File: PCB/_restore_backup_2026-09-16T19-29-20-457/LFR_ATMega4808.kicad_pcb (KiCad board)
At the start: 2 copper layers, 51.7 x 63.4 mm, 49 parts, among them J1 Conn_02x02_Odd_Even, J2 Conn_02x05_Odd_Even, J3 Conn_02x02_Counter_Clockwise, J4 Conn_02x02_Counter_Clockwise, J5 Conn_02x02_Counter_Clockwise, J6 Conn_02x03_Odd_Even, Q2 NMOS, Q3 NMOS, U1 ATmega4808-A, U5 MCP1700x-330xxTO

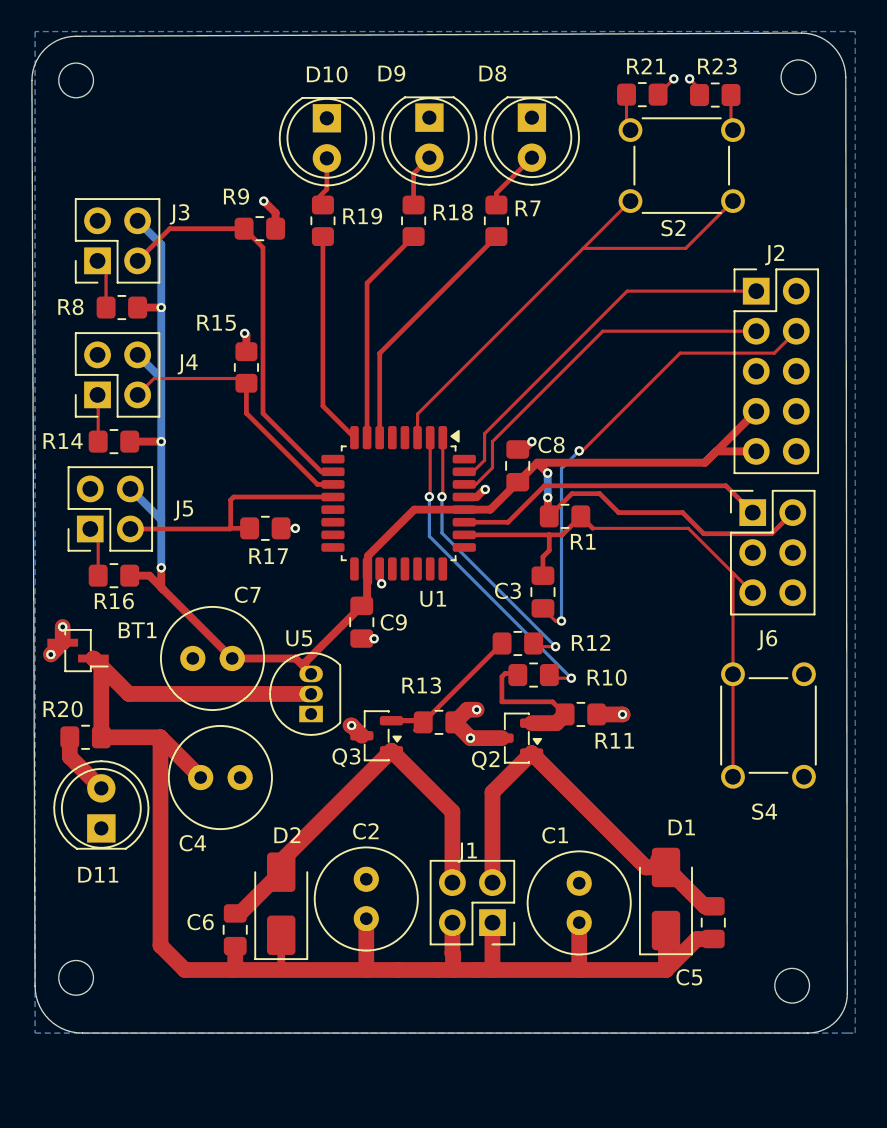
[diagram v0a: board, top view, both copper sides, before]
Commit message: Final touches, v1 is ready
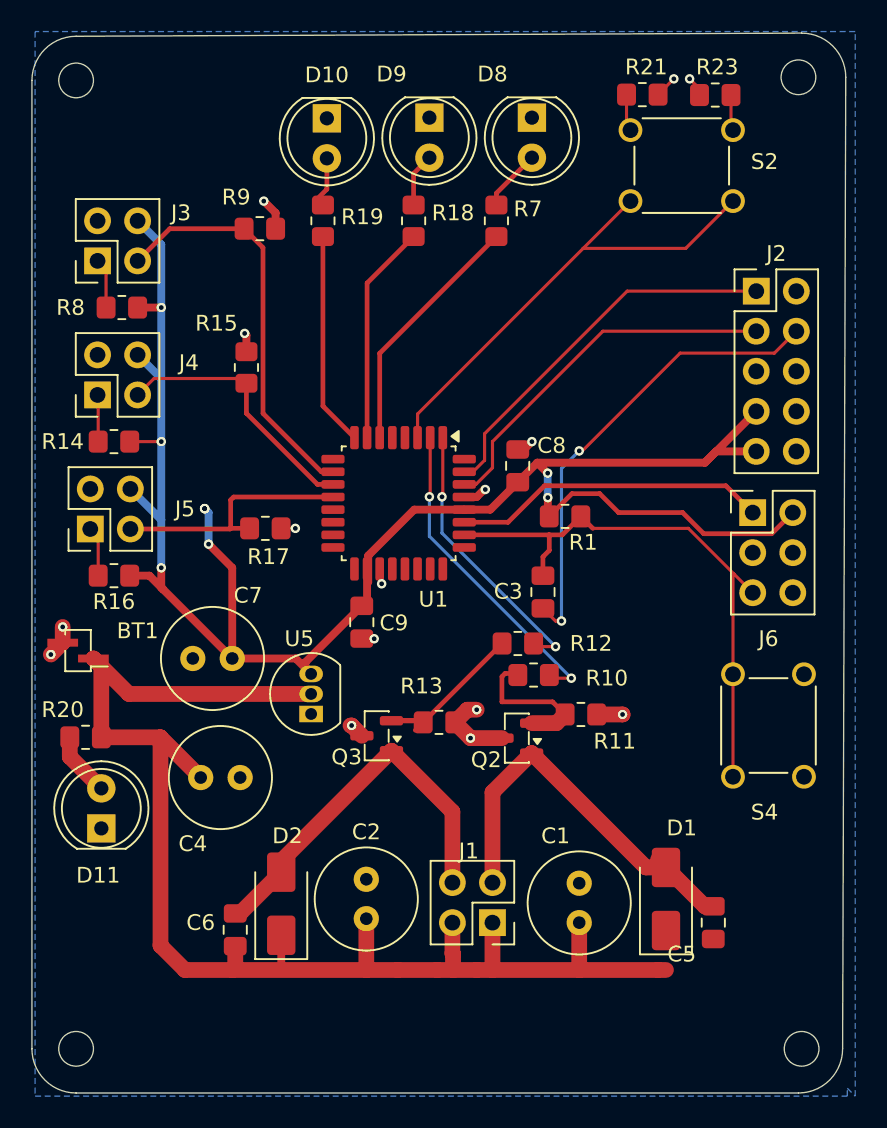
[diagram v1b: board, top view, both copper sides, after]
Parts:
- moved H4 4.50 mm to (135.6, 153.0)
- moved H3 4.04 mm to (181.6, 153.0)
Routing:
- net +3.3V: track 109.9 -> 120.2 mm, vias 5 -> 8
- net +4.8V: track 95.6 -> 89.3 mm
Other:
- board size 51.7 x 63.4 mm -> 51.6 x 67.2 mm
- board text added: "Peter Ladur Line Following Robot"
- board text removed: "LAB_A/01 B: Peter, Arinze, Antoine, Ollie"
- board text removed: "V1"
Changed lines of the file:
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@@
 		(tags "capacitor handsolder")
 		(property "Reference" "C5"
-			(at -3.5 -1.5 180)
+			(at -2 -2 180)
 			(layer "F.SilkS")
 			(effects
@@
 	(footprint "MountingHole:MountingHole_2.2mm_M2"
 		(layer "F.Cu")
-		(at 181 149)
+		(at 181.6 153)
 		(descr "Mounting Hole 2.2mm, M2, no annular, generated by kicad-footprint-generator mountinghole.py")
 		(tags "mountinghole M2")
@@
 	(footprint "MountingHole:MountingHole_2.2mm_M2"
 		(layer "F.Cu")
-		(at 135.6 148.5)
+		(at 135.6 153)
 		(descr "Mounting Hole 2.2mm, M2, no annular, generated by kicad-footprint-generator mountinghole.py")
 		(tags "mountinghole M2")
@@
 		(at 174 97)
 		(property "Reference" "S2"
-			(at -0.5 4 0)
+			(at 5.25 -0.25 0)
 			(layer "F.SilkS")
 			(effects
@@
 	(gr_line
 		(start 132.8 91.6)
-		(end 133.000002 148.999741)
+		(end 132.8 153)
 		(stroke
 			(width 0.05)
@@
 	)
 	(gr_arc
-		(start 136 152)
-		(mid 133.872653 151.127164)
-		(end 133.000002 148.999741)
+		(start 135.6 155.8)
+		(mid 133.620101 154.979899)
+		(end 132.8 153)
 		(stroke
 			(width 0.05)
@@
 	)
 	(gr_line
-		(start 136 152)
-		(end 182 152)
+		(start 135.6 155.8)
+		(end 181.4 155.8)
 		(stroke
 			(width 0.05)
@@
 		(layer "Edge.Cuts")
 	)
-	(gr_line
-		(start 184.4 91.4)
-		(end 184.5 149.5)
+	(gr_arc
+		(start 184.2 153)
+		(mid 183.379899 154.979899)
+		(end 181.4 155.8)
 		(stroke
 			(width 0.05)
@@
 		(layer "Edge.Cuts")
 	)
-	(gr_arc
-		(start 184.5 149.5)
-		(mid 183.767767 151.267767)
-		(end 182 152)
+	(gr_line
+		(start 184.4 91.4)
+		(end 184.2 153)
 		(stroke
 			(width 0.05)
@@
 		(layer "Edge.Cuts")
 	)
-	(gr_text "LAB_A/01 B: Peter, Arinze, Antoine, Ollie"
-		(at 178 150.5 0)
-		(layer "B.SilkS")
-		(effects
-			(font
-				(size 1.5 1.27)
-				(thickness 0.1875)
-			)
-			(justify left bottom mirror)
-		)
-	)
-	(gr_text "V1"
-		(at 177.5 147.5 0)
+	(gr_text "Peter Ladur\nLine Following Robot"
+		(at 182.25 147.5 0)
 		(layer "B.SilkS")
 		(effects
 			(font
-				(size 1.5 2.032)
+				(size 1.5 1.5)
 				(thickness 0.3)
 				(bold yes)
@@
 	)
 	(segment
-		(start 141 114.5)
-		(end 139 114.5)
-		(width 0.5)
-		(layer "F.Cu")
-		(net "+3.3V")
-	)
-	(segment
 		(start 145.5 128.25)
 		(end 141.125 123.875)
@@
 	)
 	(segment
+		(start 141 114.5)
+		(end 139 114.5)
+		(width 0.2)
+		(layer "F.Cu")
+		(net "+3.3V")
+	)
+	(segment
+		(start 164.8375 115.8375)
+		(end 165.5 116.5)
+		(width 0.5)
+		(layer "F.Cu")
+		(net "+3.3V")
+	)
+	(segment
 		(start 141 106)
 		(end 139.5 106)
@@
 	)
 	(segment
-		(start 164.8375 115.8375)
-		(end 165.5 116.5)
+		(start 145.5 128.25)
+		(end 145.5 122.5)
 		(width 0.5)
 		(layer "F.Cu")
@@
 	)
 	(segment
+		(start 145.5 122.5)
+		(end 144 121)
+		(width 0.5)
+		(layer "F.Cu")
+		(net "+3.3V")
+	)
+	(segment
 		(start 140.25 123)
 		(end 139 123)
@@
 	)
 	(via
+		(at 144 121)
+		(size 0.6)
+		(drill 0.3)
+		(layers "F.Cu" "B.Cu")
+		(net "+3.3V")
+	)
+	(via
+		(at 143.75 118.75)
+		(size 0.6)
+		(drill 0.3)
+		(layers "F.Cu" "B.Cu")
+		(net "+3.3V")
+	)
+	(via
 		(at 141 114.5)
 		(size 0.6)
@@
 	)
 	(via
+		(at 143.75 118.75)
+		(size 0.6)
+		(drill 0.3)
+		(layers "F.Cu" "B.Cu")
+		(net "+3.3V")
+	)
+	(via
 		(at 165.5 116.5)
 		(size 0.6)
@@
 	)
 	(segment
+		(start 144 121)
+		(end 144 119)
+		(width 0.5)
+		(layer "B.Cu")
+		(net "+3.3V")
+	)
+	(segment
 		(start 141 119.46)
 		(end 139.04 117.5)
@@
 	)
 	(segment
+		(start 144 119)
+		(end 143.75 118.75)
+		(width 0.5)
+		(layer "B.Cu")
+		(net "+3.3V")
+	)
+	(segment
 		(start 141 106)
 		(end 141 110.5)
@@
 	)
 	(segment
-		(start 159.5 147)
-		(end 159.46 146.96)
-		(width 1)
-		(layer "F.Cu")
-		(net "+4.8V")
-	)
-	(segment
-		(start 161 148)
-		(end 162 148)
+		(start 167.5 148)
+		(end 172.5 148)
 		(width 1)
 		(layer "F.Cu")
@@
 	)
 	(segment
-		(start 173 148)
-		(end 173 145.5)
+		(start 159.5 147)
+		(end 159.46 146.96)
 		(width 1)
 		(layer "F.Cu")
@@
 	)
 	(segment
-		(start 174.9625 146.0375)
-		(end 176 146.0375)
+		(start 161 148)
+		(end 162 148)
 		(width 1)
 		(layer "F.Cu")
@@
 	)
 	(segment
-		(start 167.5 148)
-		(end 173 148)
-		(width 1)
-		(layer "F.Cu")
-		(net "+4.8V")
-	)
-	(segment
 		(start 162 148)
 		(end 167.5 148)
@@
 	)
 	(segment
-		(start 173 148)
-		(end 174.9625 146.0375)
-		(width 1)
-		(layer "F.Cu")
-		(net "+4.8V")
-	)
-	(segment
 		(start 137.2 133.25)
 		(end 137.2 128.75)
@@
 	)
 	(segment
+		(start 172.5 148)
+		(end 173 148)
+		(width 1)
+		(layer "F.Cu")
+		(net "+4.8V")
+	)
+	(segment
 		(start 140.95 133.25)
 		(end 143.5 135.8)
@@
 		(polygon
 			(pts
-				(xy 185 88.5) (xy 133 88.5) (xy 133 152) (xy 184.5 152) (xy 185 152)
+				(xy 185 88.5) (xy 133 88.5) (xy 133 156) (xy 184.5 156) (xy 184.5 155.5) (xy 185 156)
 			)
 		)
